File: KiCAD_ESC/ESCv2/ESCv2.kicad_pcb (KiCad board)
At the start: 2 copper layers, 14 parts, among them P1 CONN_01X02, P2 CONN_01X02, P3 CONN_01X02, Q1 Q_NMOS_DGS, Q2 Q_NMOS_DGS, U1 IR2101

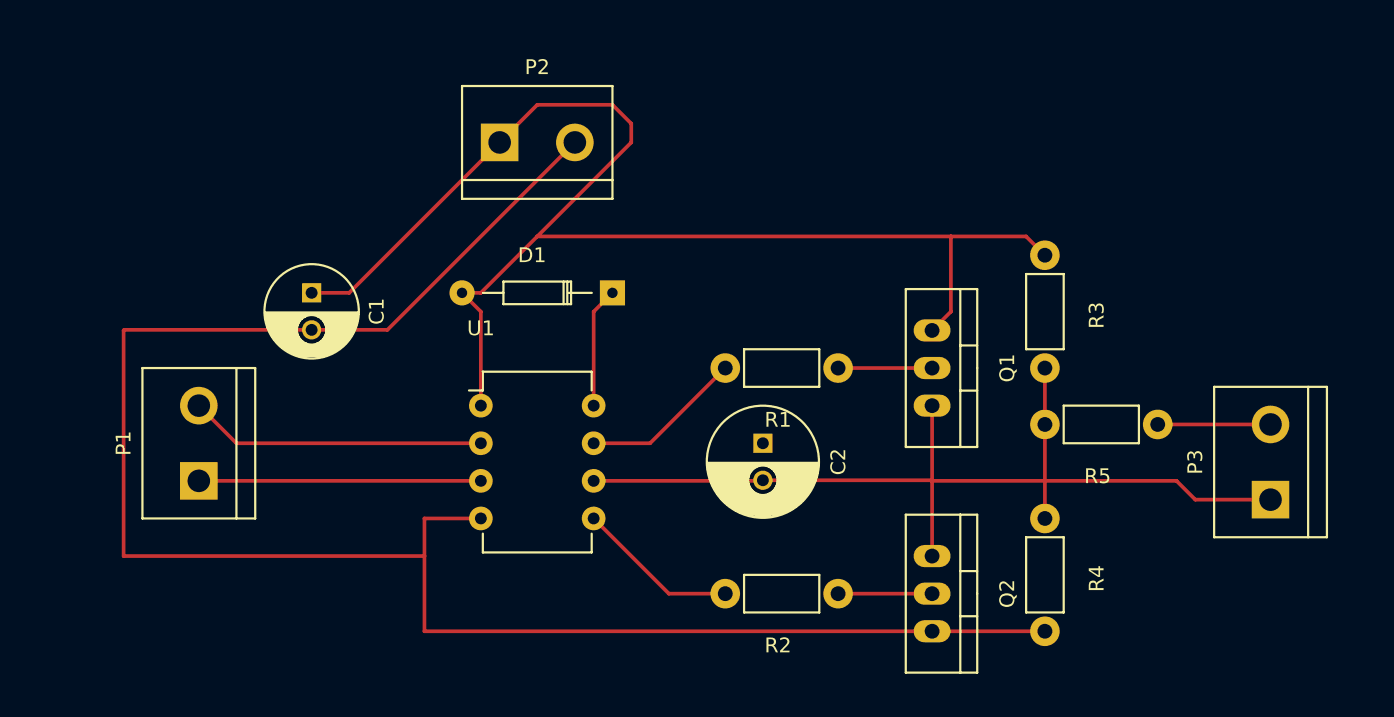
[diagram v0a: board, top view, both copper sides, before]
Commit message: kicad de mieux en mieux
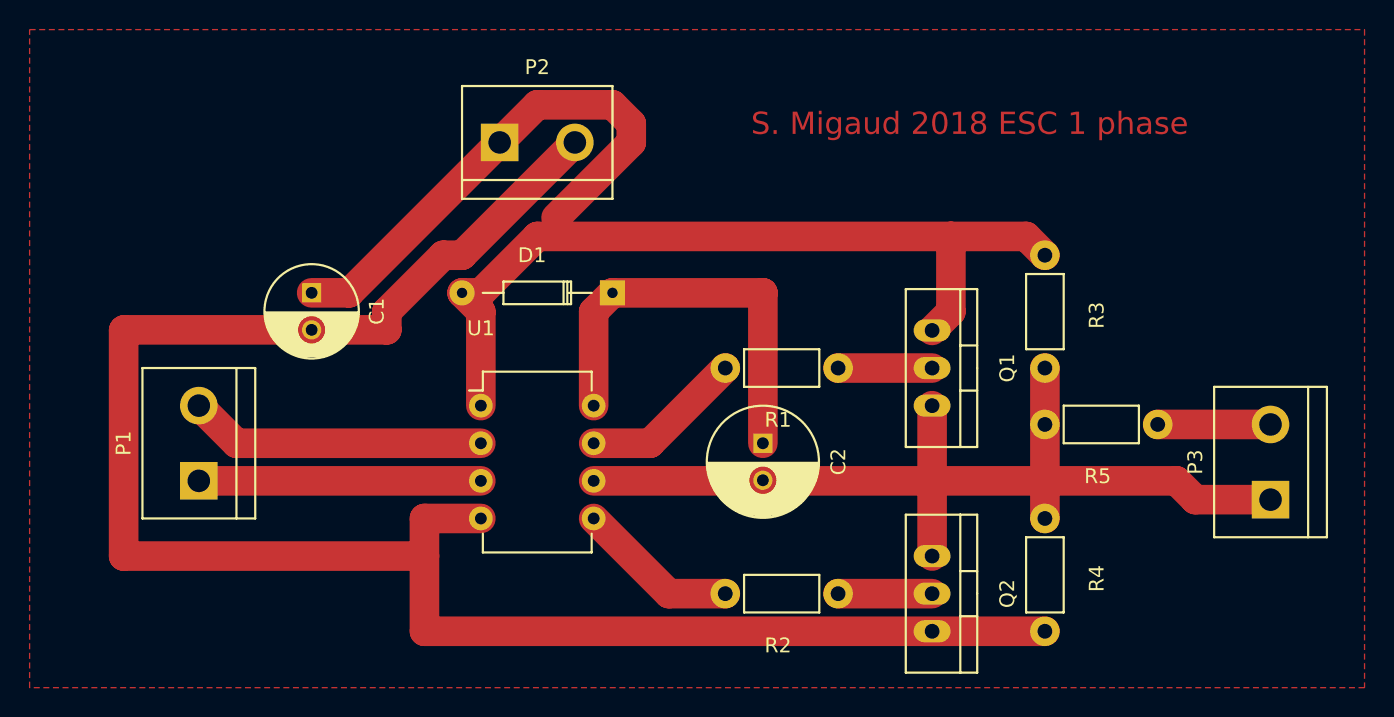
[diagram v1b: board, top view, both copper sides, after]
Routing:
- net GND: track 124.6 -> 209.2 mm
- net +12C: track 94.1 -> 175.8 mm
- net Net-(C2-Pad2): track 66.6 -> 133.2 mm
- net Net-(C2-Pad1): track 8.14 -> 30.3 mm
- net Net-(R2-Pad2): track 11.0 -> 14.8 mm
- net Net-(R1-Pad2): track 11.0 -> 14.8 mm
- net Net-(P1-Pad2): track 20.1 -> 23.7 mm
- added copper zone on F.Cu, net GND
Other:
- board text added: "S. Migaud 2018 ESC 1 phase"
